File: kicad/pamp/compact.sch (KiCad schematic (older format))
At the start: 79 parts, among them J1 input, J2 Conn_01x02_Female, J3 output, J4 power, Q1 2SA1381F, Q10 BC546B, Q11 MJE340, Q12 2SA1381F, Q13 2SC3503F, Q14 BC546B, Q15 BC556B, Q16 IRFP240N, Q17 IRFP9240N, Q2 2SC3503F, Q3 2SA1381F, Q4 2SC3503F, Q5 BC550C, Q6 BC560C, Q7 BC550C, Q8 BC560C, Q9 BC556B

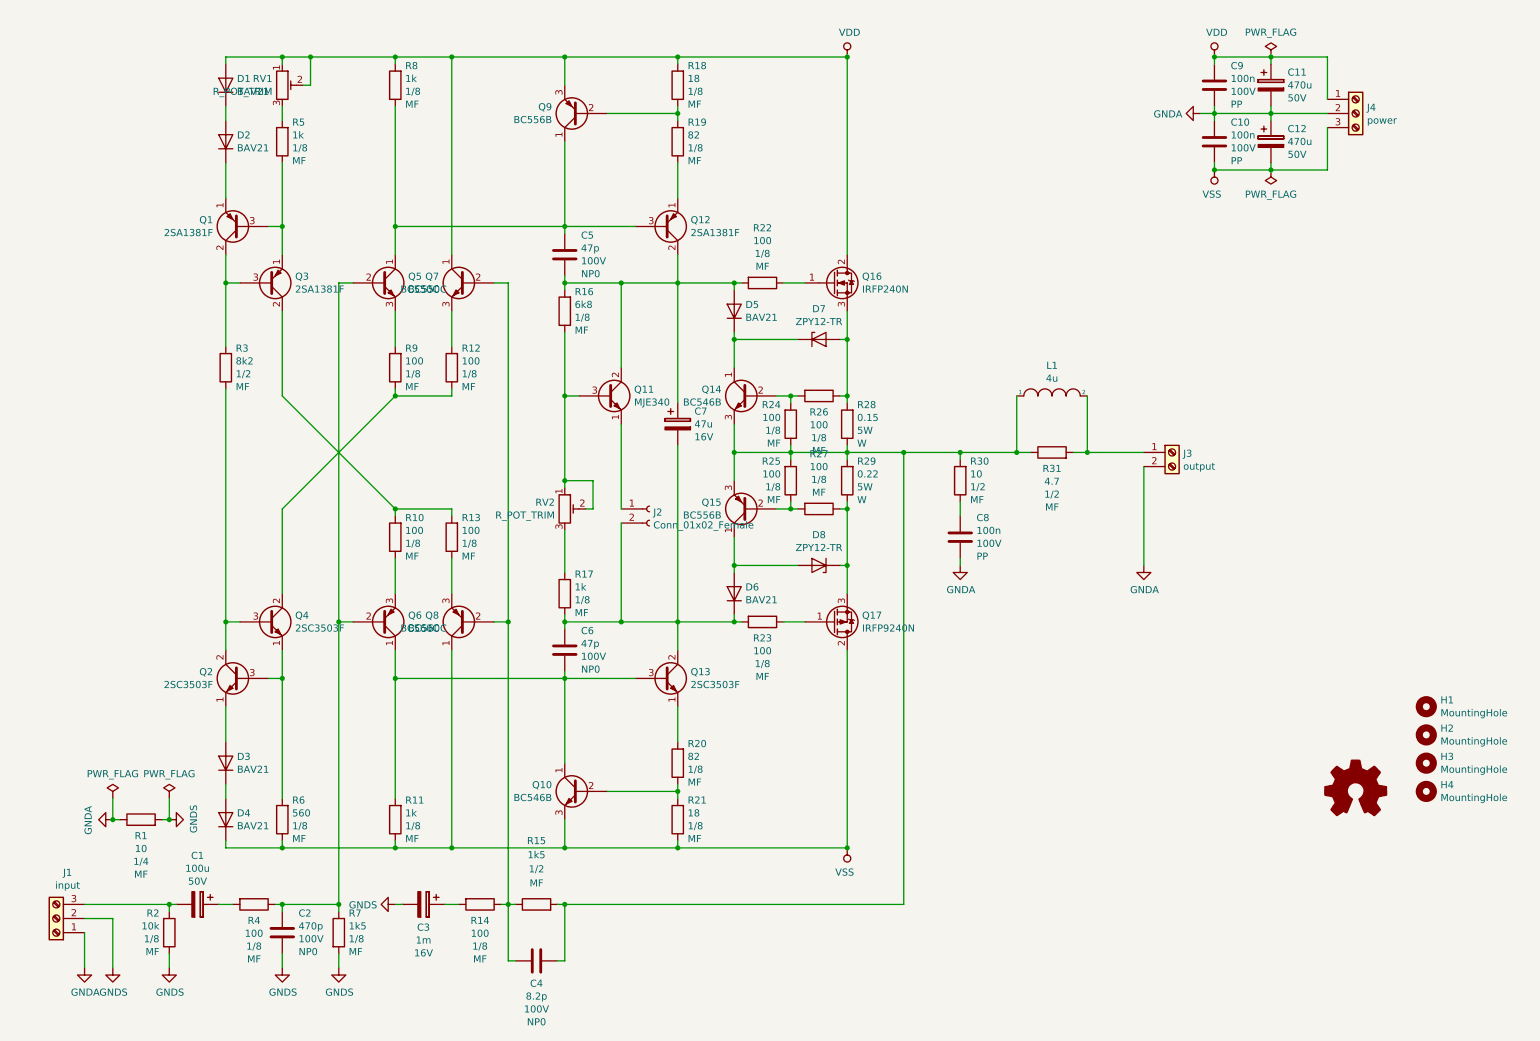
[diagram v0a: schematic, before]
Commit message: WIP: Done schematic.
Signed-off-by: Nenad Radulovic <nenad.b.radulovic@gmail.com>
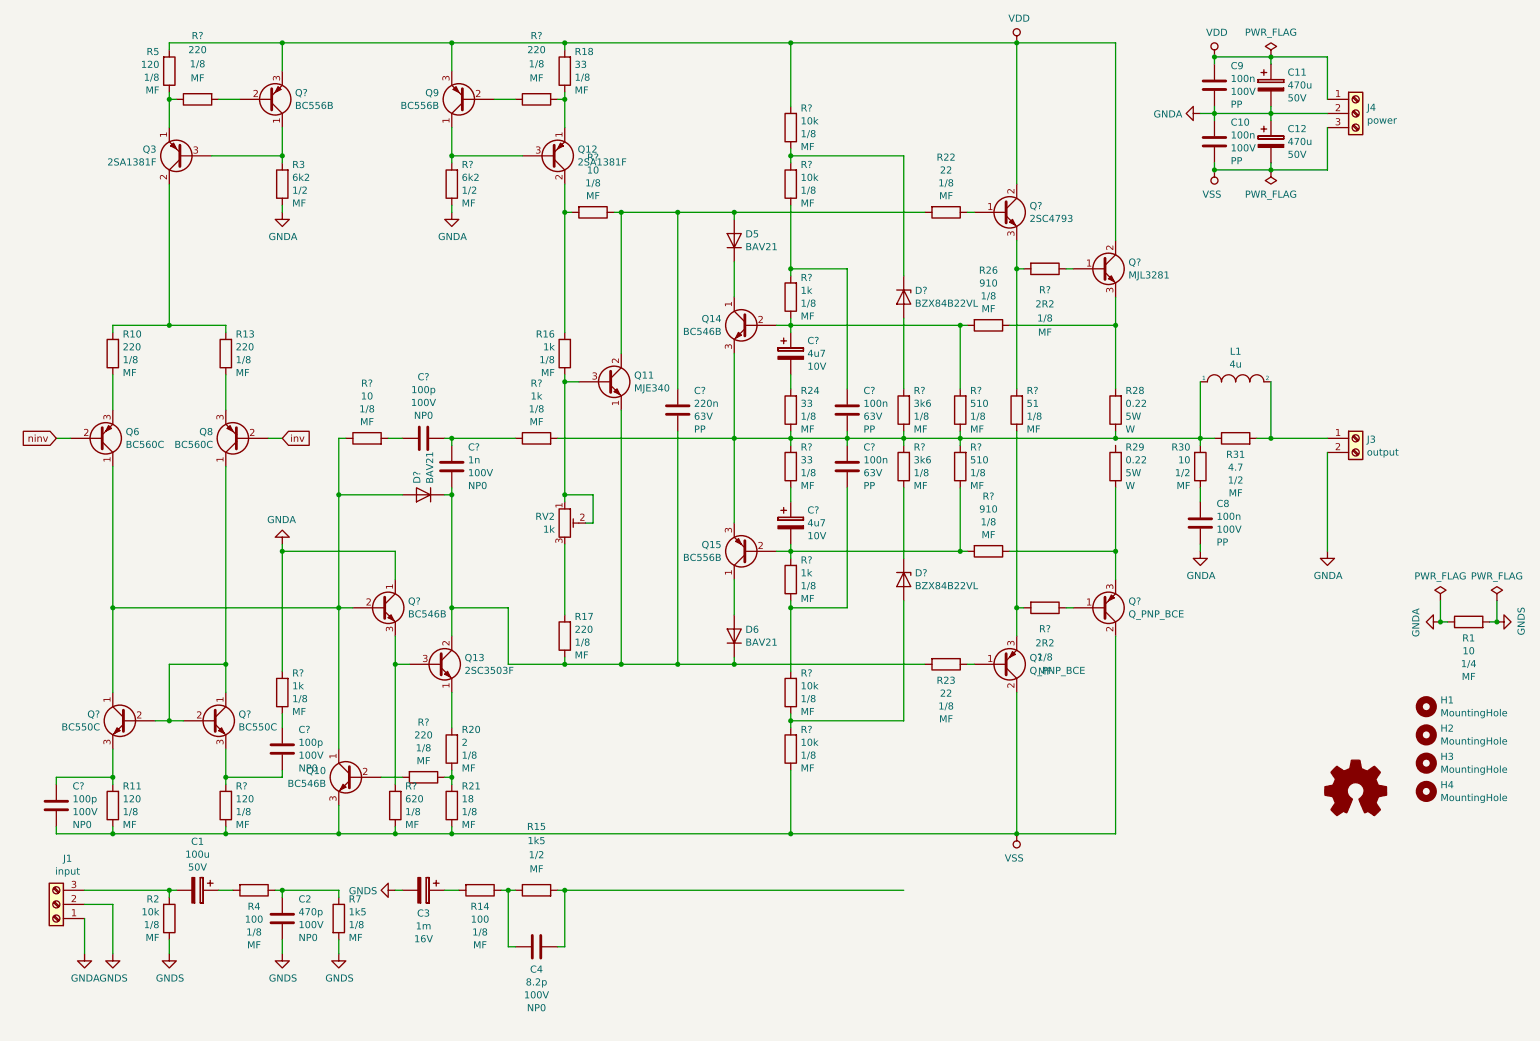
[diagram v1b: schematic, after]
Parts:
- removed C5, C6: 47p, Capacitor_THT:C_Disc_D3.0mm_W2.0mm_P2.50mm, symbol Device:C
- removed C7: 47u, Capacitor_THT:CP_Radial_D8.0mm_P2.50mm, symbol Device:CP
- removed D1, D2, D3, D4: BAV21, Diode_THT:D_DO-41_SOD81_P7.62mm_Horizontal, symbol Device:D
- removed D7, D8: ZPY12-TR, Diode_THT:D_DO-41_SOD81_P10.16mm_Horizontal, symbol Device:D_Zener
- removed J2: Conn_01x02_Female, Connector_PinHeader_2.54mm:PinHeader_1x02_P2.54mm_Vertical, symbol Connector:Conn_01x02_Female
- removed Q1: 2SA1381F, Package_TO_SOT_THT:TO-126-3_Vertical, symbol Device:Q_PNP_ECB
- removed Q16: IRFP240N, Package_TO_SOT_THT:TO-247-3_Vertical, symbol Transistor_FET:IRF540N
- removed Q17: IRFP9240N, Package_TO_SOT_THT:TO-247-3_Vertical, symbol Transistor_FET:IRF9540N
- removed Q2, Q4: 2SC3503F, Package_TO_SOT_THT:TO-126-3_Vertical, symbol Device:Q_NPN_ECB
- removed Q5, Q7: BC550C, Package_TO_SOT_THT:TO-92L_Inline, symbol Device:Q_NPN_CBE
- removed R12, R25, R27, R9: 100, Resistor_THT:R_Axial_DIN0207_L6.3mm_D2.5mm_P10.16mm_Horizontal, symbol Device:R
- removed R19: 82, Resistor_THT:R_Axial_DIN0207_L6.3mm_D2.5mm_P10.16mm_Horizontal, symbol Device:R
- removed R6: 560, Resistor_THT:R_Axial_DIN0207_L6.3mm_D2.5mm_P10.16mm_Horizontal, symbol Device:R
- removed R8: 1k, Resistor_THT:R_Axial_DIN0207_L6.3mm_D2.5mm_P10.16mm_Horizontal, symbol Device:R
- removed RV1: R_POT_TRIM, Potentiometer_THT:Potentiometer_ACP_CA9-V10_Vertical, symbol Device:R_POT_TRIM
- added C? (x3): 100p, Capacitor_THT:C_Disc_D8.0mm_W2.5mm_P5.00mm, symbol Device:C
- added C? (x2): 4u7, Capacitor_THT:CP_Radial_D5.0mm_P2.50mm, symbol Device:CP
- added C? (x2): 100n, Capacitor_THT:C_Rect_L7.2mm_W2.5mm_P5.00mm_FKS2_FKP2_MKS2_MKP2, symbol Device:C
- added C?: 220n, Capacitor_THT:C_Rect_L7.2mm_W4.5mm_P5.00mm_FKS2_FKP2_MKS2_MKP2, symbol Device:C
- added C?: 1n, Capacitor_THT:C_Disc_D8.0mm_W2.5mm_P5.00mm, symbol Device:C
- added D? (x2): BZX84B22VL, Diode_THT:D_DO-41_SOD81_P7.62mm_Horizontal, symbol Device:D_Zener
- added D?: BAV21, Diode_THT:D_DO-41_SOD81_P7.62mm_Horizontal, symbol Device:D
- added Q?: 2SC4793, Package_TO_SOT_THT:TO-220-3_Vertical, symbol Device:Q_NPN_BCE
- added Q? (x2): Q_PNP_BCE, symbol Device:Q_PNP_BCE
- added Q?: BC556B, Package_TO_SOT_THT:TO-92L_Inline, symbol Device:Q_PNP_CBE
- added Q? (x2): BC550C, Package_TO_SOT_THT:TO-92L_Inline, symbol Device:Q_NPN_CBE
- added Q?: BC546B, Package_TO_SOT_THT:TO-92L_Inline, symbol Device:Q_NPN_CBE
- added Q?: MJL3281, Package_TO_SOT_THT:TO-220-3_Vertical, symbol Device:Q_NPN_BCE
- added R? (x3): 220, Resistor_THT:R_Axial_DIN0207_L6.3mm_D2.5mm_P10.16mm_Horizontal, symbol Device:R
- added R? (x2): 10, Resistor_THT:R_Axial_DIN0207_L6.3mm_D2.5mm_P10.16mm_Horizontal, symbol Device:R
- added R?: 120, Resistor_THT:R_Axial_DIN0207_L6.3mm_D2.5mm_P10.16mm_Horizontal, symbol Device:R
- added R?: 51, Resistor_THT:R_Axial_DIN0207_L6.3mm_D2.5mm_P10.16mm_Horizontal, symbol Device:R
- added R? (x4): 1k, Resistor_THT:R_Axial_DIN0207_L6.3mm_D2.5mm_P10.16mm_Horizontal, symbol Device:R
- added R? (x4): 10k, Resistor_THT:R_Axial_DIN0207_L6.3mm_D2.5mm_P10.16mm_Horizontal, symbol Device:R
- added R? (x2): 3k6, Resistor_THT:R_Axial_DIN0207_L6.3mm_D2.5mm_P10.16mm_Horizontal, symbol Device:R
- added R?: 620, Resistor_THT:R_Axial_DIN0207_L6.3mm_D2.5mm_P10.16mm_Horizontal, symbol Device:R
- added R?: 6k2, Resistor_THT:R_Axial_DIN0411_L9.9mm_D3.6mm_P12.70mm_Horizontal, symbol Device:R
- added R?: 33, Resistor_THT:R_Axial_DIN0207_L6.3mm_D2.5mm_P10.16mm_Horizontal, symbol Device:R
- added R? (x2): 510, Resistor_THT:R_Axial_DIN0207_L6.3mm_D2.5mm_P10.16mm_Horizontal, symbol Device:R
- added R?: 910, Resistor_THT:R_Axial_DIN0207_L6.3mm_D2.5mm_P10.16mm_Horizontal, symbol Device:R
- added R? (x2): 2R2, Resistor_THT:R_Axial_DIN0207_L6.3mm_D2.5mm_P10.16mm_Horizontal, symbol Device:R
- R10, R13: value 100 -> 220
- R11, R5: value 1k -> 120
- R16: value 6k8 -> 1k
- R17: value 1k -> 220
- R18: value 18 -> 33
- R20: value 82 -> 2
- R22, R23: value 100 -> 22
- R24: value 100 -> 33
- R26: value 100 -> 910
- R28: value 0.15 -> 0.22
- R3: value 8k2 -> 6k2
- RV2: value R_POT_TRIM -> 1k
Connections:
- net GNDA: now also R3.1, Q?.1 (C), R?.1, R?.2
- net VDD: now also R5.2, Q?.2 (C), Q?.2 (C), Q?.3 (E), R?.2
- net VSS: now also C?.2, Q?.2 (C), Q?.2 (C), R?.1, R?.1, R?.1; no longer Q8.1 (C)
- net at R22.1: now also Q?.1 (B)
- net at R26.1, R28.2: now also Q?.3 (E)
- net at D5.2 (A), Q11.2 (C), R22.2: now also C?.1, R?.1; no longer Q12.2 (C), R16.2
- net at L1.1, Q14.3 (E), Q15.3 (E)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: now also C?.1, C?.2, R?.1, R?.1, R?.2, R?.2, R?.2, R?.2; no longer C4.1, R15.2, R29.2
- net at R29.1: now also Q?.3 (E), R?.1
- net at R23.1: now also Q?.1 (B)
- net at D6.1 (K), Q13.2 (C), R17.1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: now also Q11.1 (E), C?.1, C?.2, D?.1 (K)
- net at Q14.2 (B), R26.2: now also C?.1, R?.1, R?.2; no longer R24.2
- net at Q15.2 (B): now also C?.2, R?.1, R?.2, R?.2
- net at Q10.1 (C), Q6.1 (C): now also D?.2 (A), Q?.1 (C), Q?.2 (B), R?.1; no longer Q13.3 (B), R11.2
- net at R20.1, R21.2: now also R?.1; no longer Q10.2 (B)
- net at Q12.1 (E): now also R18.1, R?.2
- net at Q12.3 (B), Q9.1 (C): now also R?.2
- net at Q9.2 (B): now also R?.1; no longer R18.1
- net at C4.2, R14.1, R15.1: no longer Q8.2 (B)
- net at C2.2, R4.1, R7.1: no longer Q6.2 (B)
- net at Q3.1 (E), R5.1: now also R?.1
- net at Q3.3 (B), R3.2: now also Q?.1 (C)
- new net: C?.2, R24.2
- new net: Q12.2 (C), R16.2, R?.2
- new net: Q13.3 (B), Q?.3 (E), R?.2
- new net: Q10.2 (B), R?.2
- new net: Q8.1 (C), Q?.1 (C), Q?.2 (B), Q?.2 (B)
- new net: C?.1, Q?.3 (E), R11.2
- new net: Q?.3 (E), R?.2, R?.2
- new net: Q?.3 (E), R?.1, R?.2
- new net: Q?.2 (B), R?.2
- new net: C?.2, Q?.3 (E), R?.2
- new net: C?.1, R?.1 (x2)
- new net: C?.1, R?.1, R?.2
- new net: D?.1 (K), R?.1, R?.2
- new net: C?.1, C?.2, R?.1
- new net: C?.2, R?.2
- new net: C4.1, R15.2
- new net: D?.2 (A), R?.2
- new net: D?.1 (K), R?.1
- new net: D?.2 (A), R?.1, R?.2
- new net: C?.2, R?.1, R?.2
- new net: Q?.1 (B), R?.1 (x2)
- new net inv: Q8.2 (B)
- new net ninv: Q6.2 (B)
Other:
- moved on the sheet: C1, C2, C3, C4, C8, D5, D6, J1, J3, L1, Q10, Q11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
